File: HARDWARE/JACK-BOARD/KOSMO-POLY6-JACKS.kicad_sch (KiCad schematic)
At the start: 30 parts, among them J1 RAMP_OUT0, J10 RAMP_OUT3, J11 PULSE_OUT3, J12 GATE_OUT3, J13 RAMP_OUT4, J14 PULSE_OUT4, J15 GATE_OUT4, J16 RAMP_OUT5, J17 PULSE_OUT5, J18 GATE_OUT5, J2 PULSE_OUT0, J3 GATE_OUT0, J4 RAMP_OUT1, J5 PULSE_OUT1, J6 GATE_OUT1, J7 RAMP_OUT2, J8 PULSE_OUT2, J9 GATE_OUT2

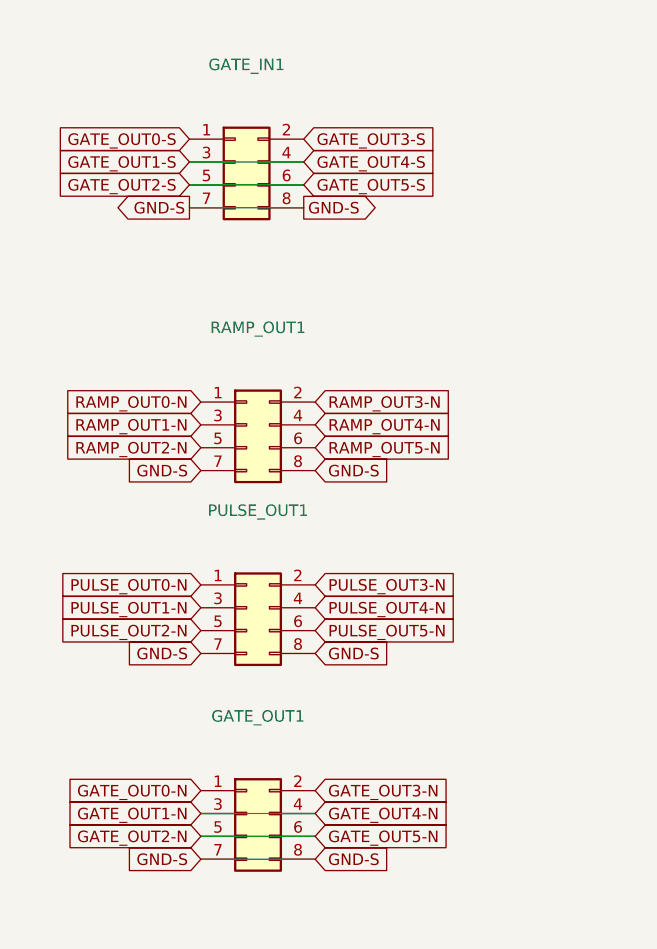
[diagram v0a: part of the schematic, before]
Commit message: holidaysync
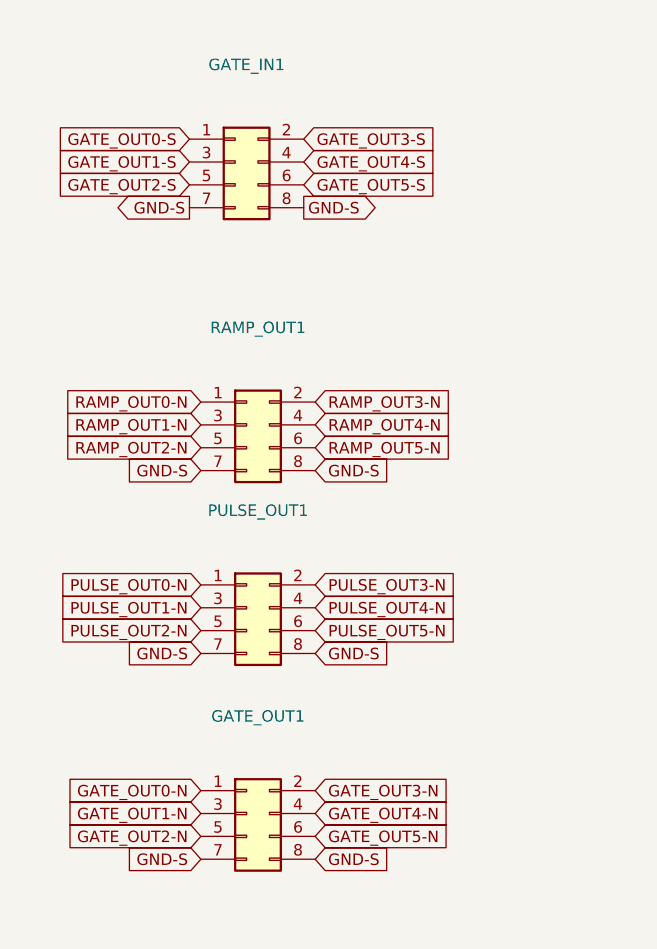
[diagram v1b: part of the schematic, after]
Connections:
- net GATE_OUT1-N: no longer GATE_OUT1.4 (Pin_4), J15.TN
- net GATE_OUT1-S: no longer GATE_IN1.4 (Pin_4), J15.T
- net GATE_OUT2-N: no longer GATE_OUT1.6 (Pin_6), J18.TN
- net GATE_OUT2-S: no longer GATE_IN1.6 (Pin_6), J18.T
- new net GATE_OUT4-N: GATE_OUT1.4 (Pin_4), J15.TN
- new net GATE_OUT4-S: GATE_IN1.4 (Pin_4), J15.T
- new net GATE_OUT5-N: GATE_OUT1.6 (Pin_6), J18.TN
- new net GATE_OUT5-S: GATE_IN1.6 (Pin_6), J18.T
